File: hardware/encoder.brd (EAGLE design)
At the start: 30.5 x 21.3 mm, 11 parts

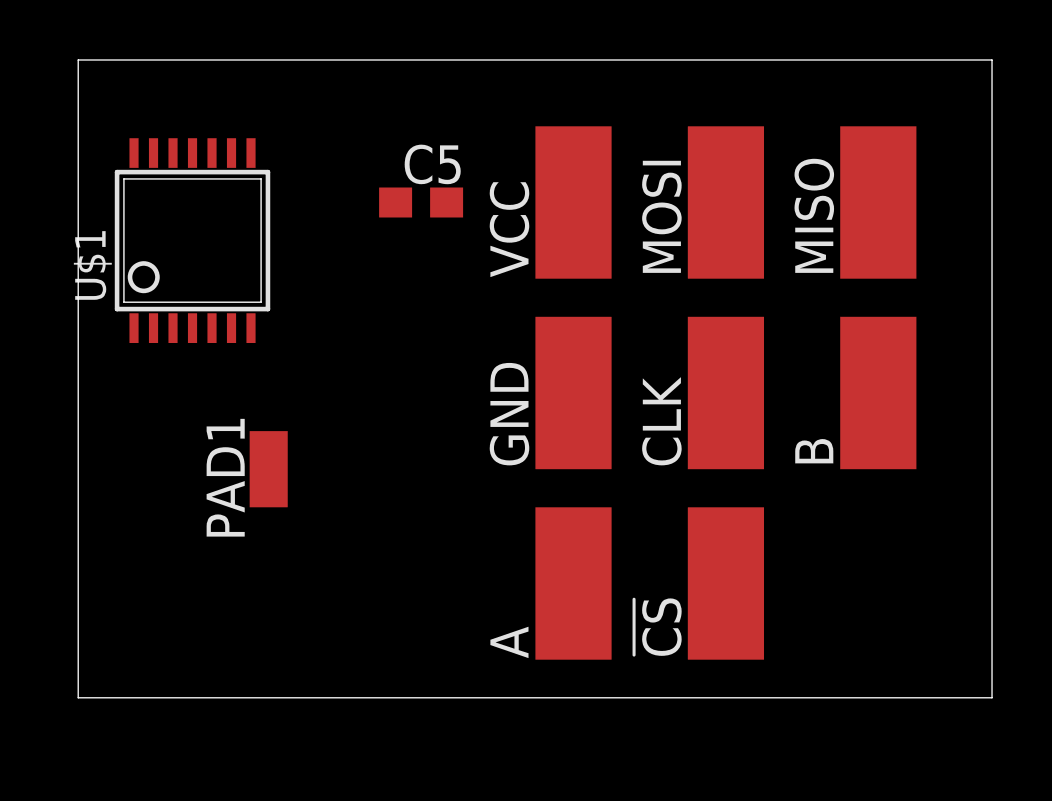
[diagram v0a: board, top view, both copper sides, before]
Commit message: encoder brd
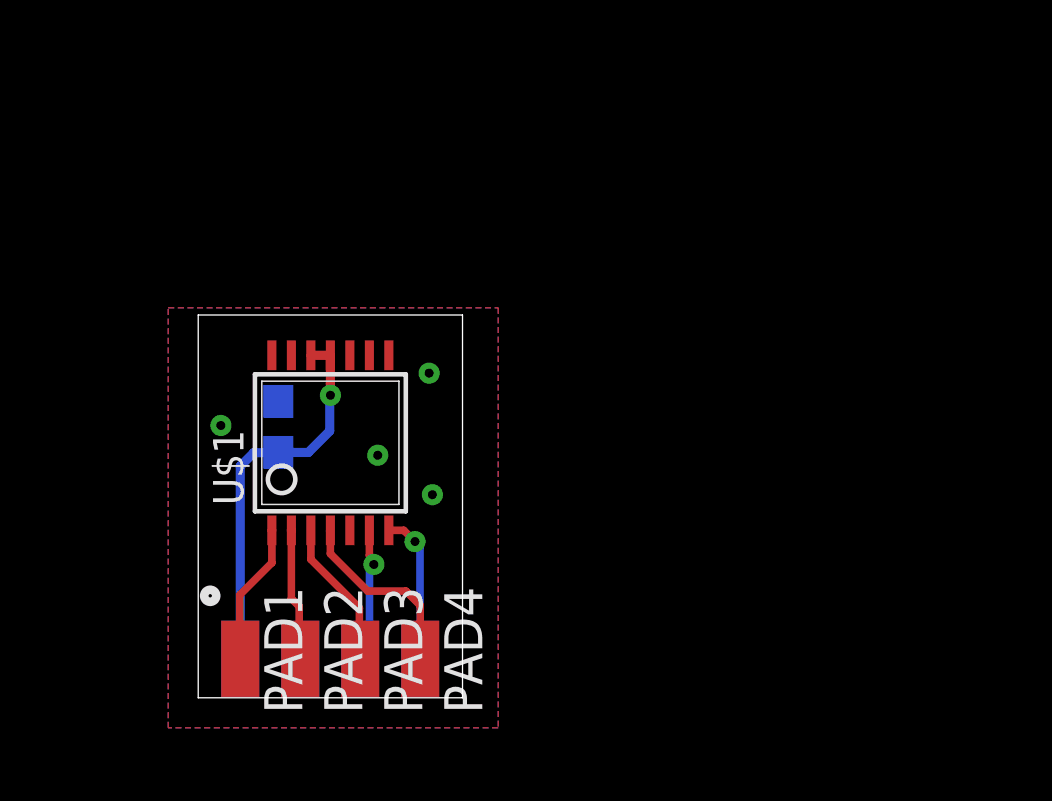
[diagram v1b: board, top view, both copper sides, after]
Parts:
- removed !CS, A, B, CLK, GND, MISO, MOSI, VCC: (no value), wirepad:SMD2,54-5,08
- added PAD2, PAD3, PAD4, PAD5, PAD6, PAD7, PAD8: (no value), wirepad:SMD1,27-2,54
- moved C5 8.87 mm to (6.67, 9.03), flipped to the bottom, turned to 90 degrees
- moved U$1 8.16 mm to (8.40, 8.50)
- moved PAD1 6.39 mm to (5.40, 1.30), turned to 180 degrees
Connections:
- removed net N$38: !CS.1, U$1.1
- removed net N$39: CLK.1, U$1.2
- removed net N$40: MISO.1, U$1.3
- removed net N$41: MOSI.1, U$1.4
- removed net N$42: A.1, U$1.7
- removed net N$43: B.1, U$1.6
- removed net N$46: C5.1, U$1.11, U$1.12, VCC.1
- new net A: PAD6.1, U$1.7
- new net B: PAD7.1, U$1.6
- new net CLK: PAD2.1, U$1.2
- new net CS: PAD1.1, U$1.1
- new net MISO: PAD3.1, U$1.3
- new net MOSI: PAD4.1, U$1.4
- new net VCC: C5.1, PAD8.1, U$1.11, U$1.12
- net GND: now also PAD5.1; no longer GND.1
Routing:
- net VCC: track 0.00 -> 13.1 mm, vias 0 -> 1
- net MOSI: track 0.00 -> 6.30 mm
- net MISO: track 0.00 -> 5.72 mm
- net A: track 0.00 -> 5.01 mm, vias 0 -> 1
- net CS: track 0.00 -> 4.74 mm
- net B: track 0.00 -> 4.72 mm, vias 0 -> 1
- net CLK: track 0.00 -> 4.41 mm
- added copper zone on layer 1, net GND
- added copper zone on layer 16, net GND
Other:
- board size 30.5 x 21.3 mm -> 8.8 x 12.8 mm
